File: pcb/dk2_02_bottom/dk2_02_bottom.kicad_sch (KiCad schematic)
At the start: 8 parts, among them J1 Conn_01x18_Pin, J2 Conn_01x18_Pin, U1 Pico

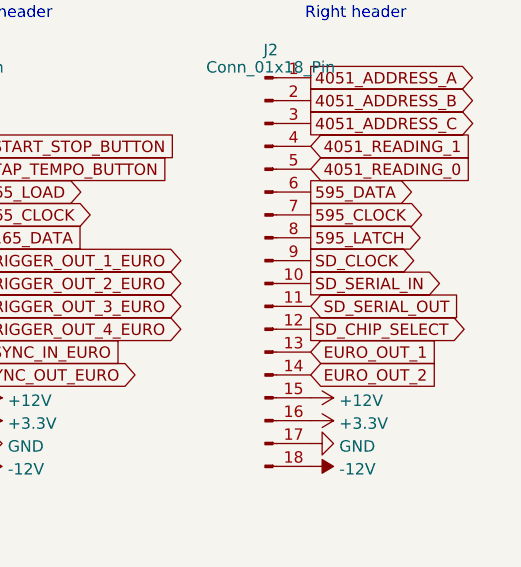
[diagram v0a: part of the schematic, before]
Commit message: done for the week, started routing
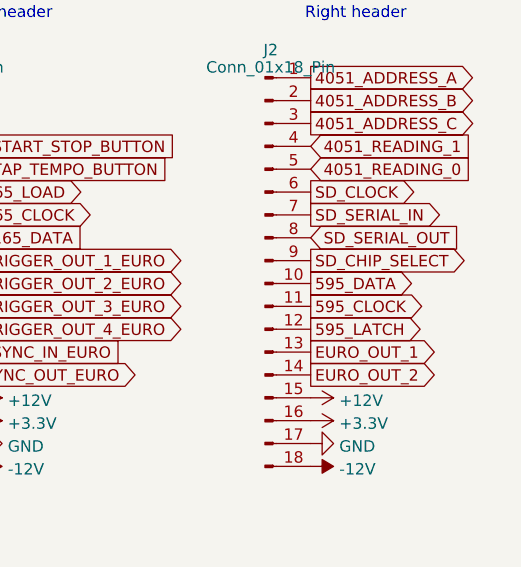
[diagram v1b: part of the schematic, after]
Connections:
- net 595_CLOCK: now also J2.11 (Pin_11); no longer J2.7 (Pin_7)
- net 595_DATA: now also J2.10 (Pin_10); no longer J2.6 (Pin_6)
- net 595_LATCH: now also J2.12 (Pin_12); no longer J2.8 (Pin_8)
- net SD_CHIP_SELECT: now also J2.9 (Pin_9); no longer J2.12 (Pin_12)
- net SD_CLOCK: now also J2.6 (Pin_6); no longer J2.9 (Pin_9)
- net SD_SERIAL_IN: now also J2.7 (Pin_7); no longer J2.10 (Pin_10)
- net SD_SERIAL_OUT: now also J2.8 (Pin_8); no longer J2.11 (Pin_11)
